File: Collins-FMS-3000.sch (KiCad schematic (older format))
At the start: 23 parts, among them U2 MCP23017_SO, U3 MCP23017_SO, U4 IS31FL3733B

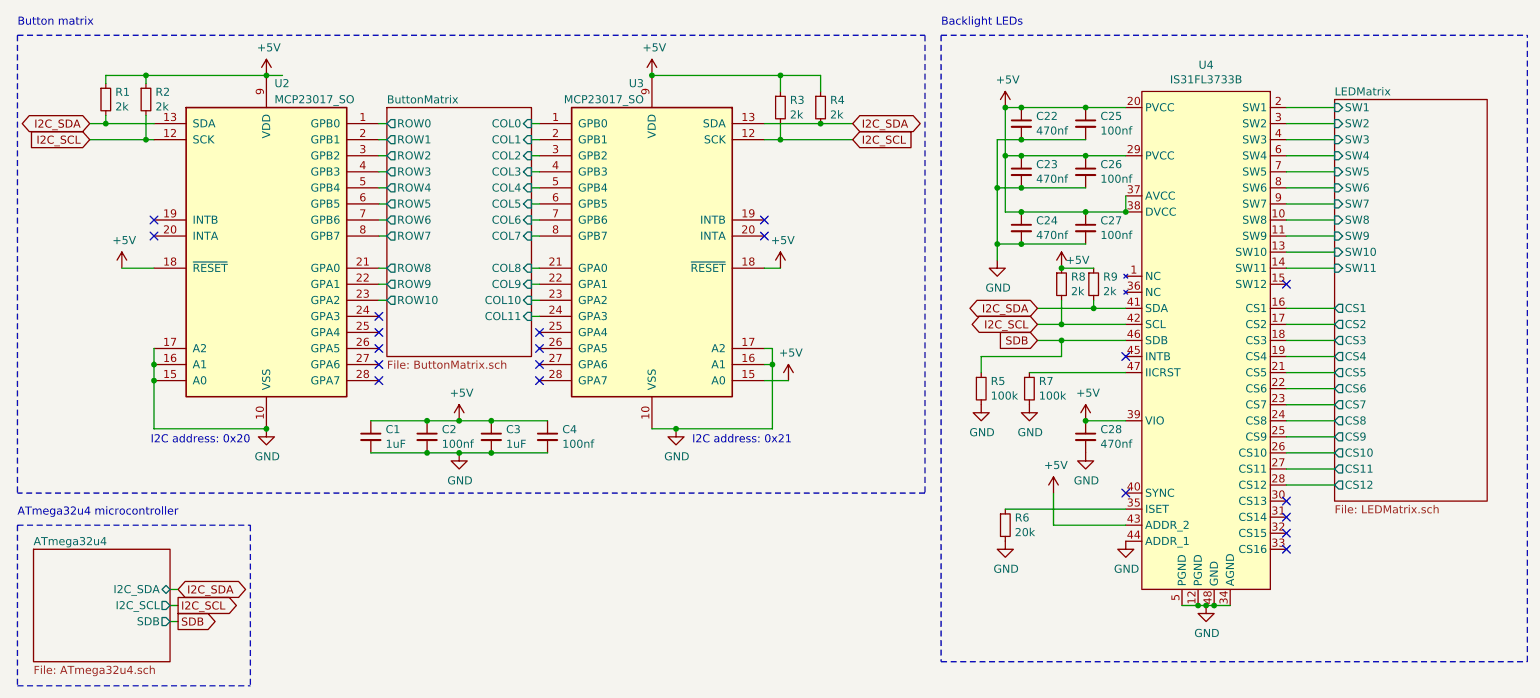
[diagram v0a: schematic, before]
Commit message: Fully routed
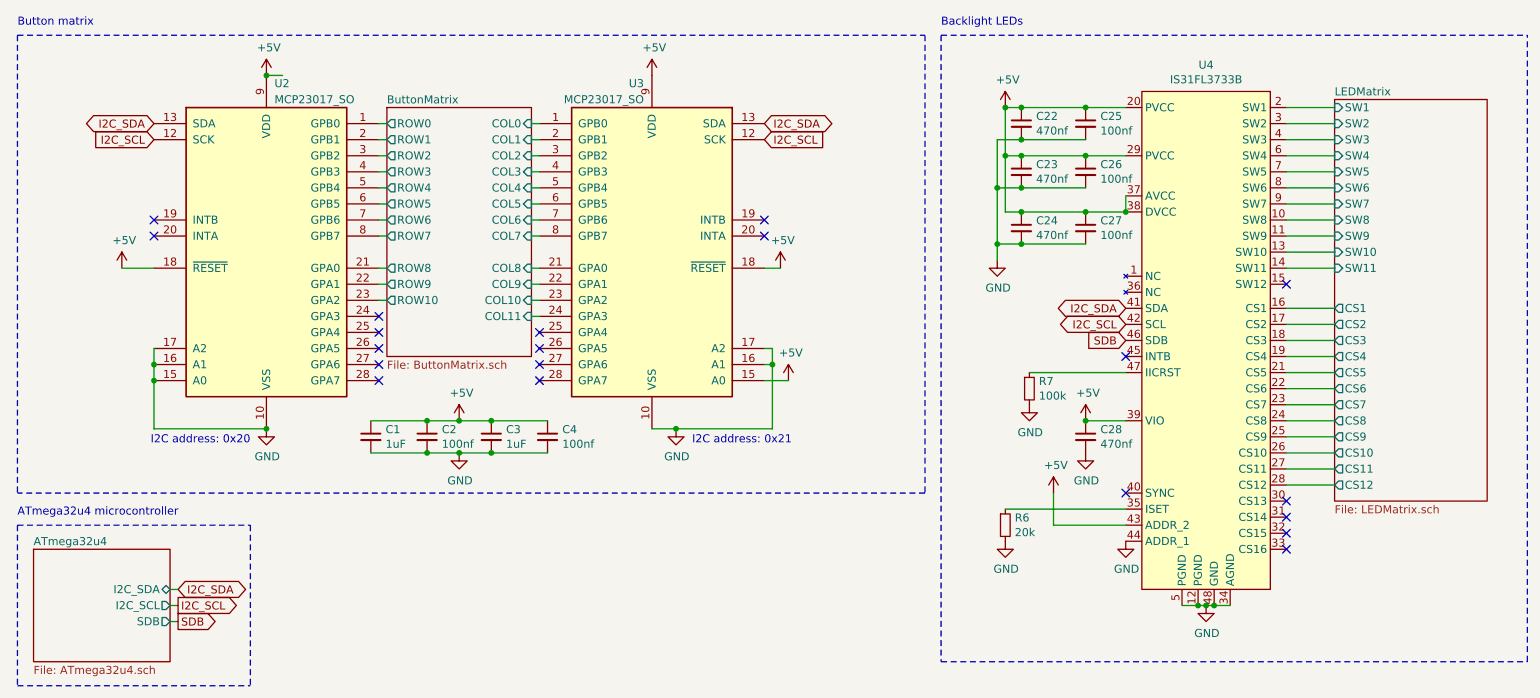
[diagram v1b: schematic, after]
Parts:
- removed R1, R2, R3, R4, R8, R9: 2k, Resistor_SMD:R_0805_2012Metric_Pad1.20x1.40mm_HandSolder, symbol Device:R_Small
- removed R5: 100k, Resistor_SMD:R_0402_1005Metric, symbol Device:R_Small
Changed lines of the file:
@@
 	1    0    0    -1
 $EndComp
-Text GLabel 1000 1200 0    50   BiDi ~ 0
+Text GLabel 1400 1200 0    50   BiDi ~ 0
 I2C_SDA
-Text GLabel 1000 1300 0    50   Input ~ 0
+Text GLabel 1400 1300 0    50   Input ~ 0
 I2C_SCL
 NoConn ~ 1400 1800
@@
 $EndComp
 Connection ~ 2100 900
-Text GLabel 5750 1200 2    50   BiDi ~ 0
+Text GLabel 5200 1200 2    50   BiDi ~ 0
 I2C_SDA
-Text GLabel 5750 1300 2    50   Input ~ 0
+Text GLabel 5200 1300 2    50   Input ~ 0
 I2C_SCL
 $Comp
@@
 Wire Wire Line
 	5200 2100 5300 2100
-Connection ~ 4500 900
 NoConn ~ 3800 2500
 NoConn ~ 3800 2600
@@
 Wire Wire Line
 	3300 3250 3100 3250
-$Comp
-L Device:R_Small R1
-U 1 1 618D9439
-P 1100 1050
-F 0 "R1" H 1159 1096 50  0000 L CNN
-F 1 "2k" H 1159 1005 50  0000 L CNN
-F 2 "Resistor_SMD:R_0805_2012Metric_Pad1.20x1.40mm_HandSolder" H 1100 1050 50  0001 C CNN
-F 3 "~" H 1100 1050 50  0001 C CNN
-	1    1100 1050
-	1    0    0    -1
-$EndComp
-$Comp
-L Device:R_Small R2
-U 1 1 618D97E0
-P 1350 1050
-F 0 "R2" H 1409 1096 50  0000 L CNN
-F 1 "2k" H 1409 1005 50  0000 L CNN
-F 2 "Resistor_SMD:R_0805_2012Metric_Pad1.20x1.40mm_HandSolder" H 1350 1050 50  0001 C CNN
-F 3 "~" H 1350 1050 50  0001 C CNN
-	1    1350 1050
-	1    0    0    -1
-$EndComp
-Wire Wire Line
-	1350 1300 1350 1150
-Wire Wire Line
-	1100 1200 1100 1150
-Wire Wire Line
-	1100 1200 1000 1200
-Wire Wire Line
-	1100 950  1100 900
-Wire Wire Line
-	1100 900  1350 900
-Wire Wire Line
-	1350 950  1350 900
-Connection ~ 1350 900
-Wire Wire Line
-	1350 900  2100 900
-Wire Wire Line
-	1400 1300 1350 1300
 Wire Wire Line
 	2100 900  2200 900
-Wire Wire Line
-	1350 1300 1000 1300
-Connection ~ 1350 1300
-Wire Wire Line
-	1100 1200 1400 1200
-Connection ~ 1100 1200
-$Comp
-L Device:R_Small R3
-U 1 1 618ED4A8
-P 5300 1100
-F 0 "R3" H 5359 1146 50  0000 L CNN
-F 1 "2k" H 5359 1055 50  0000 L CNN
-F 2 "Resistor_SMD:R_0805_2012Metric_Pad1.20x1.40mm_HandSolder" H 5300 1100 50  0001 C CNN
-F 3 "~" H 5300 1100 50  0001 C CNN
-	1    5300 1100
-	1    0    0    -1
-$EndComp
-$Comp
-L Device:R_Small R4
-U 1 1 618EDA4E
-P 5550 1100
-F 0 "R4" H 5609 1146 50  0000 L CNN
-F 1 "2k" H 5609 1055 50  0000 L CNN
-F 2 "Resistor_SMD:R_0805_2012Metric_Pad1.20x1.40mm_HandSolder" H 5550 1100 50  0001 C CNN
-F 3 "~" H 5550 1100 50  0001 C CNN
-	1    5550 1100
-	1    0    0    -1
-$EndComp
-Wire Wire Line
-	5200 1300 5300 1300
-Wire Wire Line
-	5300 1300 5300 1200
-Wire Wire Line
-	5300 1000 5300 900
-Connection ~ 5300 900
-Wire Wire Line
-	5300 900  4500 900
-Wire Wire Line
-	5550 900  5550 1000
-Wire Wire Line
-	5300 900  5550 900
-Wire Wire Line
-	5550 1200 5750 1200
-Connection ~ 5550 1200
-Wire Wire Line
-	5300 1300 5750 1300
-Connection ~ 5300 1300
 $Comp
 L power:+5V #PWR0103
@@
 $EndComp
 NoConn ~ 7450 3500
-$Comp
-L Device:R_Small R9
-U 1 1 61A0BFB6
-P 7250 2200
-F 0 "R9" H 7309 2246 50  0000 L CNN
-F 1 "2k" H 7309 2155 50  0000 L CNN
-F 2 "Resistor_SMD:R_0805_2012Metric_Pad1.20x1.40mm_HandSolder" H 7250 2200 50  0001 C CNN
-F 3 "~" H 7250 2200 50  0001 C CNN
-	1    7250 2200
-	1    0    0    -1
-$EndComp
-Wire Wire Line
-	7450 2350 7250 2350
-$Comp
-L Device:R_Small R8
-U 1 1 61A12756
-P 7050 2200
-F 0 "R8" H 7109 2246 50  0000 L CNN
-F 1 "2k" H 7109 2155 50  0000 L CNN
-F 2 "Resistor_SMD:R_0805_2012Metric_Pad1.20x1.40mm_HandSolder" H 7050 2200 50  0001 C CNN
-F 3 "~" H 7050 2200 50  0001 C CNN
-	1    7050 2200
-	1    0    0    -1
-$EndComp
-Wire Wire Line
-	7250 2300 7250 2350
-Wire Wire Line
-	7250 2100 7050 2100
-$Comp
-L power:+5V #PWR012
-U 1 1 61A250CA
-P 7050 2100
-F 0 "#PWR012" H 7050 1950 50  0001 C CNN
-F 1 "+5V" H 7150 2150 50  0000 C CNN
-F 2 "" H 7050 2100 50  0001 C CNN
-F 3 "" H 7050 2100 50  0001 C CNN
-	1    7050 2100
-	1    0    0    -1
-$EndComp
-Connection ~ 7050 2100
-Wire Wire Line
-	7450 2450 7050 2450
-Wire Wire Line
-	7050 2450 7050 2300
-Wire Wire Line
-	7250 2350 6900 2350
-Connection ~ 7250 2350
-Wire Wire Line
-	7050 2450 6900 2450
-Connection ~ 7050 2450
-Text GLabel 6900 2350 0    50   BiDi ~ 0
+Text GLabel 7450 2350 0    50   BiDi ~ 0
 I2C_SDA
-Text GLabel 6900 2450 0    50   BiDi ~ 0
+Text GLabel 7450 2450 0    50   BiDi ~ 0
 I2C_SCL
 NoConn ~ 7450 2650
@@
 $EndComp
 Connection ~ 7950 4200
-Wire Wire Line
-	7450 2550 7050 2550
-Text GLabel 6900 2550 0    50   Input ~ 0
+Text GLabel 7450 2550 0    50   Input ~ 0
 SDB
-$Comp
-L Device:R_Small R5
-U 1 1 61A7BE7A
-P 6550 2850
-F 0 "R5" H 6609 2896 50  0000 L CNN
-F 1 "100k" H 6609 2805 50  0000 L CNN
-F 2 "Resistor_SMD:R_0402_1005Metric" H 6550 2850 50  0001 C CNN
-F 3 "~" H 6550 2850 50  0001 C CNN
-	1    6550 2850
-	1    0    0    -1
-$EndComp
-Wire Wire Line
-	7050 2550 7050 2650
-Wire Wire Line
-	7050 2650 6550 2650
-Wire Wire Line
-	6550 2650 6550 2750
-Connection ~ 7050 2550
-Wire Wire Line
-	7050 2550 6900 2550
-$Comp
-L power:GND #PWR06
-U 1 1 61A8402C
-P 6550 2950
-F 0 "#PWR06" H 6550 2700 50  0001 C CNN
-F 1 "GND" H 6555 2777 50  0000 C CNN
-F 2 "" H 6550 2950 50  0001 C CNN
-F 3 "" H 6550 2950 50  0001 C CNN
-	1    6550 2950
-	1    0    0    -1
-$EndComp
 $Comp
 L Device:R_Small R6
@@
 Wire Notes Line
 	550  650  550  3500
-Wire Wire Line
-	5200 1200 5550 1200
 $EndSCHEMATC
